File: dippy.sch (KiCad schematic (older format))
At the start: 20 parts, among them J1 Conn_01x02_Female, J2 Screw_Terminal_01x03, J3 Screw_Terminal_01x04, U1 ATmega328P-PU, U2 RFM95W-915S2, U3 MCP1700-3302E_SOT23, Y1 Crystal_GND2

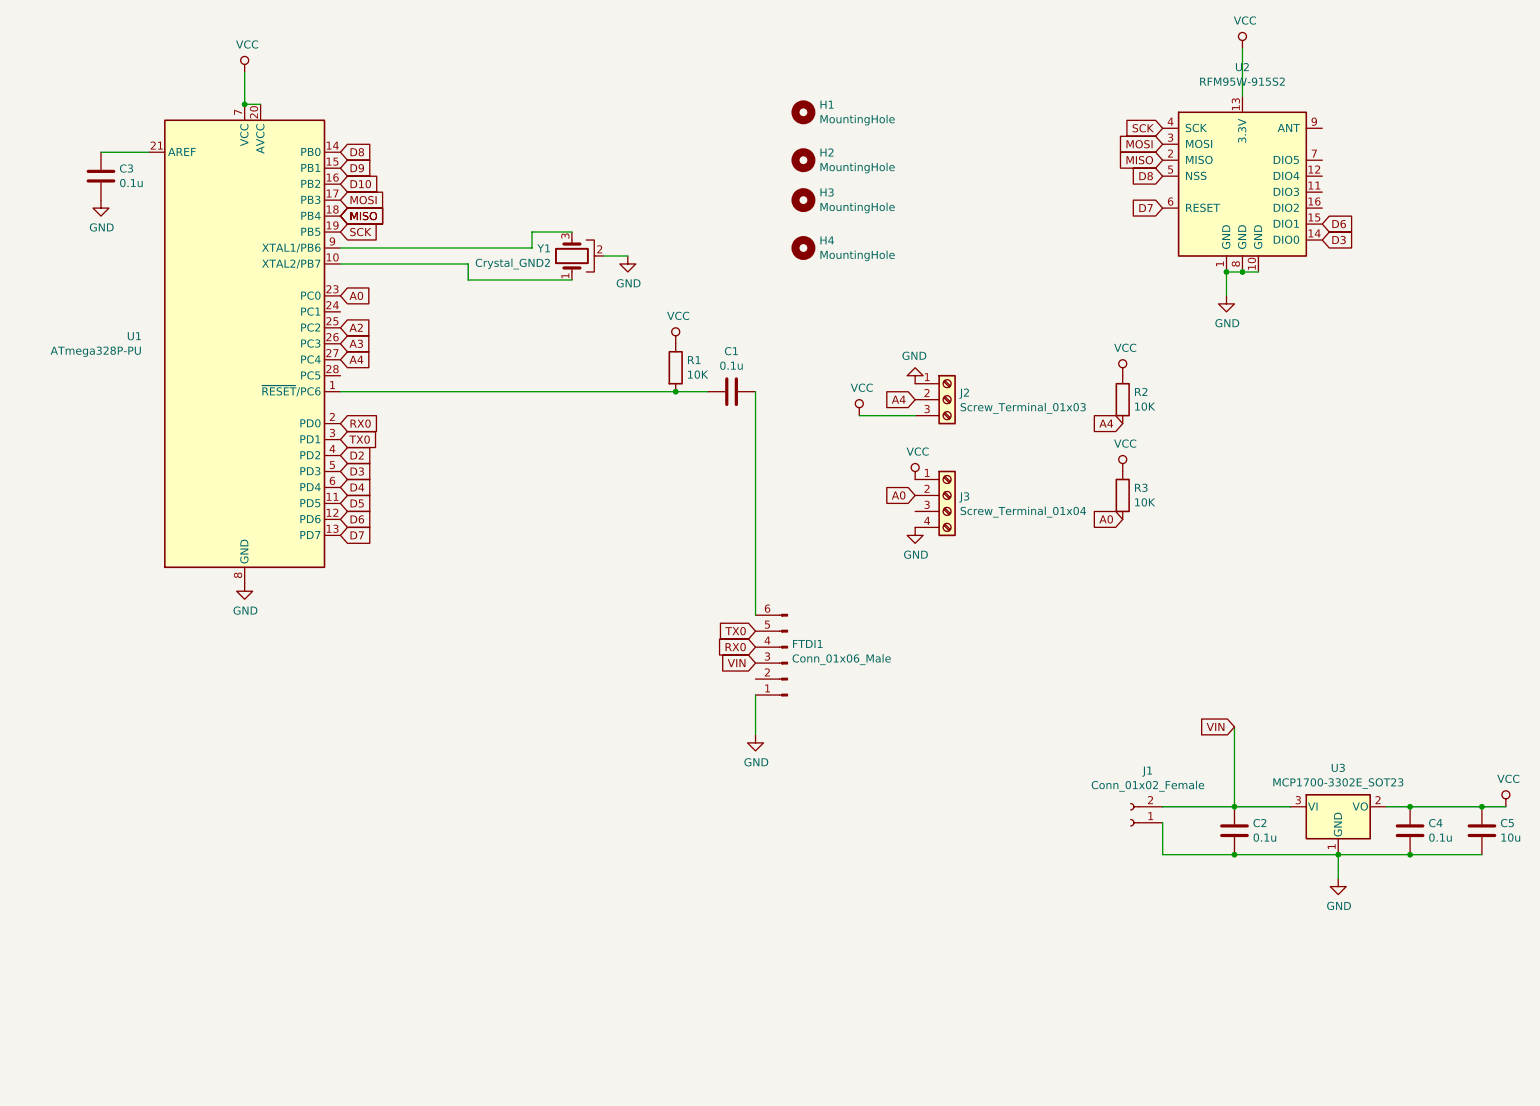
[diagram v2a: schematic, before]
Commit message: update
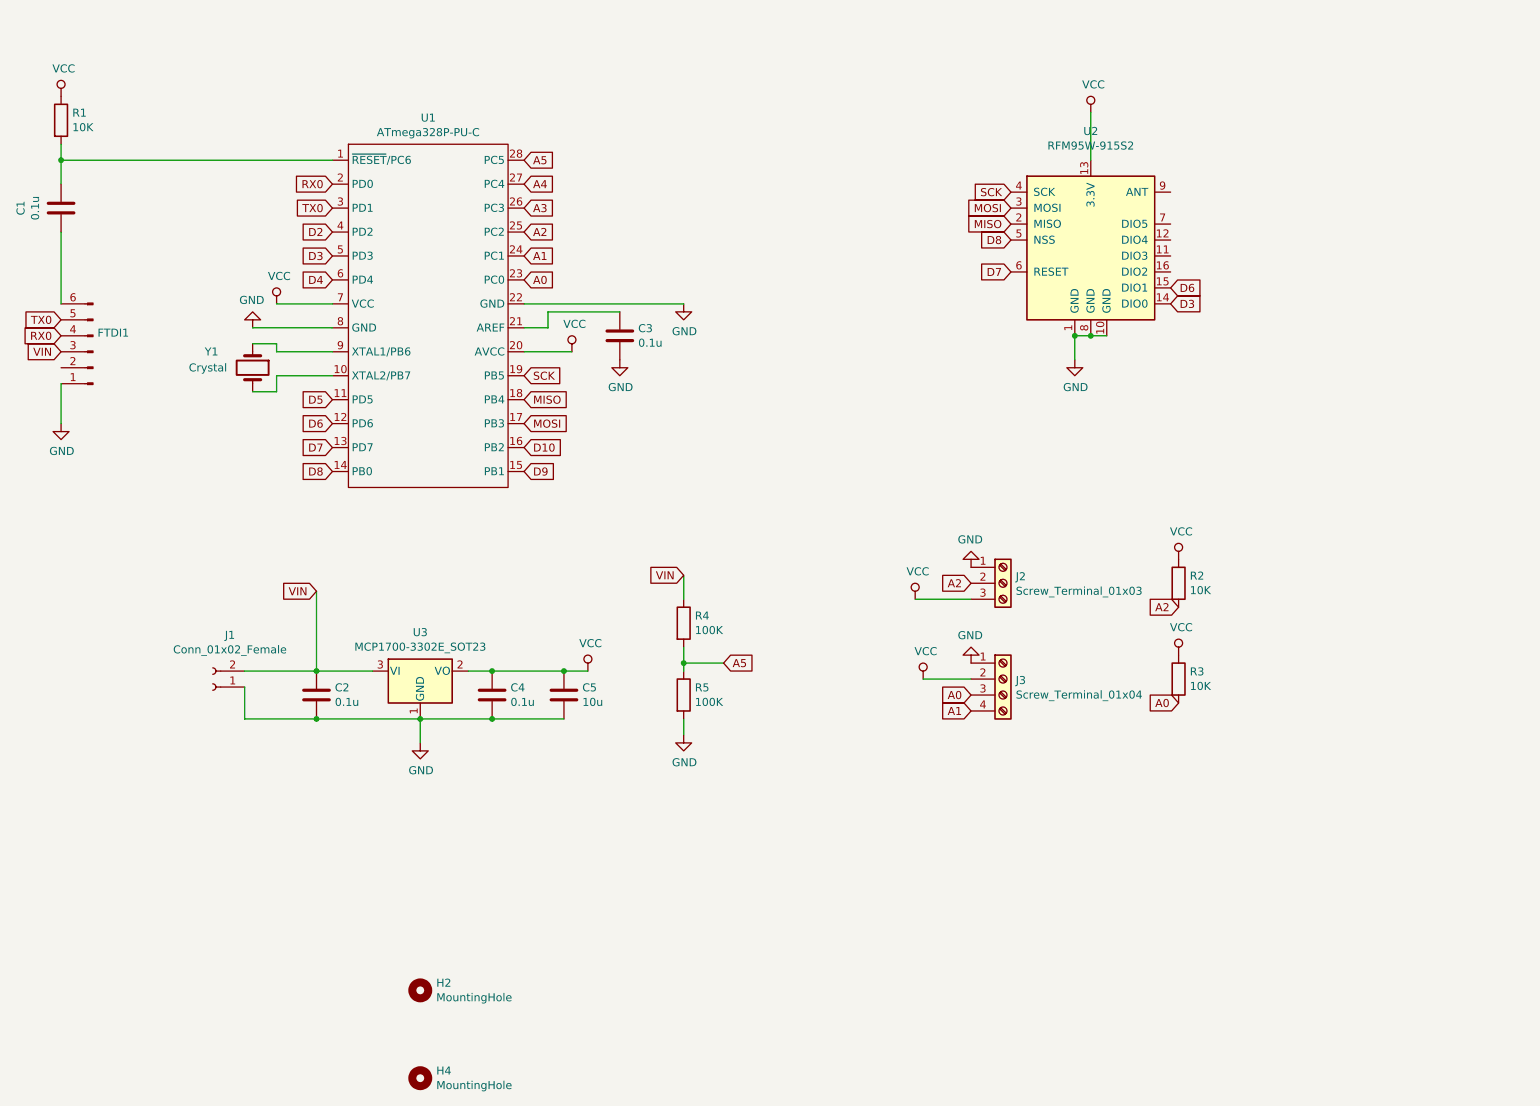
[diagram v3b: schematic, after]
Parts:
- removed H1, H3: MountingHole, MountingHole:MountingHole_2.7mm_M2.5, symbol Mechanical:MountingHole
- removed U1: ATmega328P-PU, Package_DIP:DIP-28_W7.62mm, symbol MCU_Microchip_ATmega:ATmega328P-PU
- removed Y1: Crystal_GND2, Connector_PinSocket_2.54mm:PinSocket_1x03_P2.54mm_Vertical, symbol Device:Crystal_GND2
- added R4: 100K, Resistor_THT:R_Axial_DIN0207_L6.3mm_D2.5mm_P7.62mm_Horizontal, symbol Device:R
- added R5: 100K, Resistor_THT:R_Axial_DIN0207_L6.3mm_D2.5mm_P2.54mm_Vertical, symbol Device:R
- added U1: ATmega328P-PU-C, Package_DIP:DIP-28_W7.62mm, symbol atmega328p-pu-c:ATmega328P-PU-C
- added Y1: Crystal, Crystal:Resonator-2Pin_W10.0mm_H5.0mm, symbol Device:Crystal
- C1: footprint Capacitor_THT:C_Disc_D3.0mm_W1.6mm_P2.50mm -> Capacitor_THT:C_Disc_D4.7mm_W2.5mm_P5.00mm
- R1: footprint Resistor_THT:R_Axial_DIN0207_L6.3mm_D2.5mm_P2.54mm_Vertical -> Resistor_THT:R_Axial_DIN0207_L6.3mm_D2.5mm_P5.08mm_Vertical
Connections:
- net A0: now also J3.3 (Pin_3), U1.23 (PC0); no longer J3.2 (Pin_2)
- net A2: now also J2.2 (Pin_2), R2.2, U1.25 (PC2)
- net A3: now also U1.26 (PC3)
- net A4: now also U1.27 (PC4); no longer J2.2 (Pin_2), R2.2
- net D10: now also U1.16 (PB2)
- net D2: now also U1.4 (PD2)
- net D3: now also U1.5 (PD3)
- net D4: now also U1.6 (PD4)
- net D5: now also U1.11 (PD5)
- net D6: now also U1.12 (PD6)
- net D7: now also U1.13 (PD7)
- net D8: now also U1.14 (PB0)
- net D9: now also U1.15 (PB1)
- net GND: now also J3.1 (Pin_1), R5.2, U1.22 (GND), U1.8 (GND); no longer J3.4 (Pin_4)
- net MISO: now also U1.18 (PB4)
- net MOSI: now also U1.17 (PB3)
- net RX0: now also U1.2 (PD0)
- net SCK: now also U1.19 (PB5)
- net TX0: now also U1.3 (PD1)
- net VCC: now also J3.2 (Pin_2), U1.20 (AVCC), U1.7 (VCC); no longer J3.1 (Pin_1)
- net VIN: now also R4.1
- net at R1.2: now also C1.1, U1.1 (~RESET~/PC6); no longer C1.2
- net at C3.1: now also U1.21 (AREF)
- net at FTDI1.6 (Pin_6): now also C1.2; no longer C1.1
- new net: U1.10 (XTAL2/PB7), Y1.2
- new net: U1.9 (XTAL1/PB6), Y1.1
- new net A1: J3.4 (Pin_4), U1.24 (PC1)
- new net A5: R4.2, R5.1, U1.28 (PC5)
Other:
- moved on the sheet: C1, C2, C3, C4, C5, FTDI1, H2, H4, J1, J2, J3, R1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
